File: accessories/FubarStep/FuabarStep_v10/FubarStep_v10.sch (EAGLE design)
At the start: 10 parts, among them IC1 7805, X1 DC21MMX

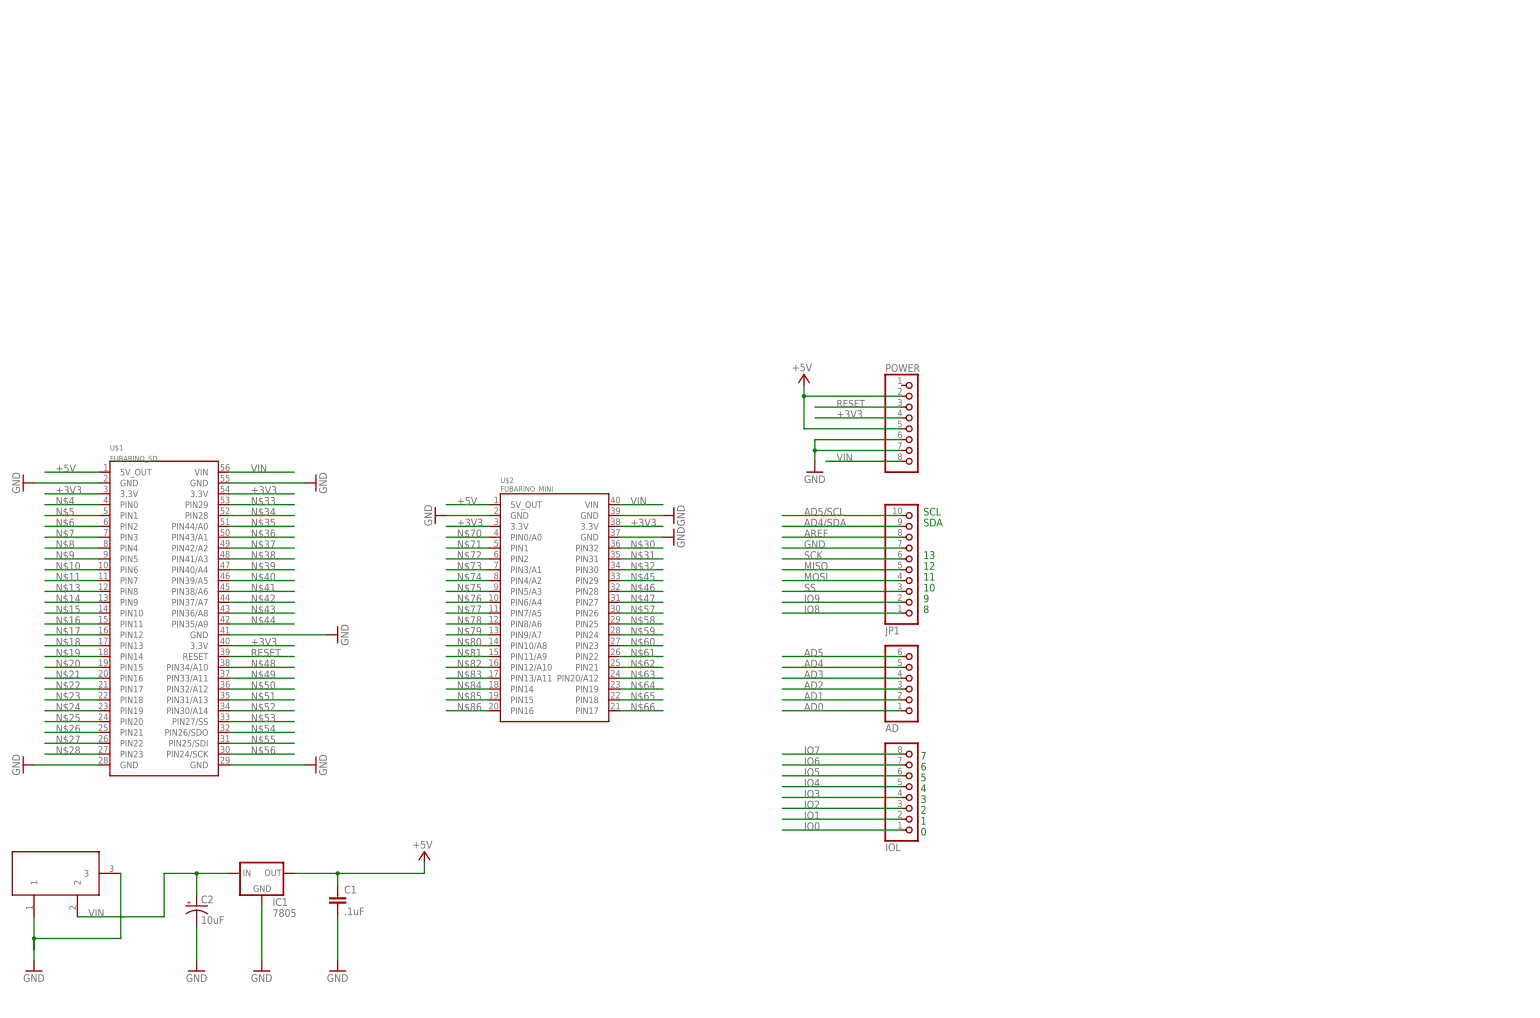
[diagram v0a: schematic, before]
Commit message: More work.
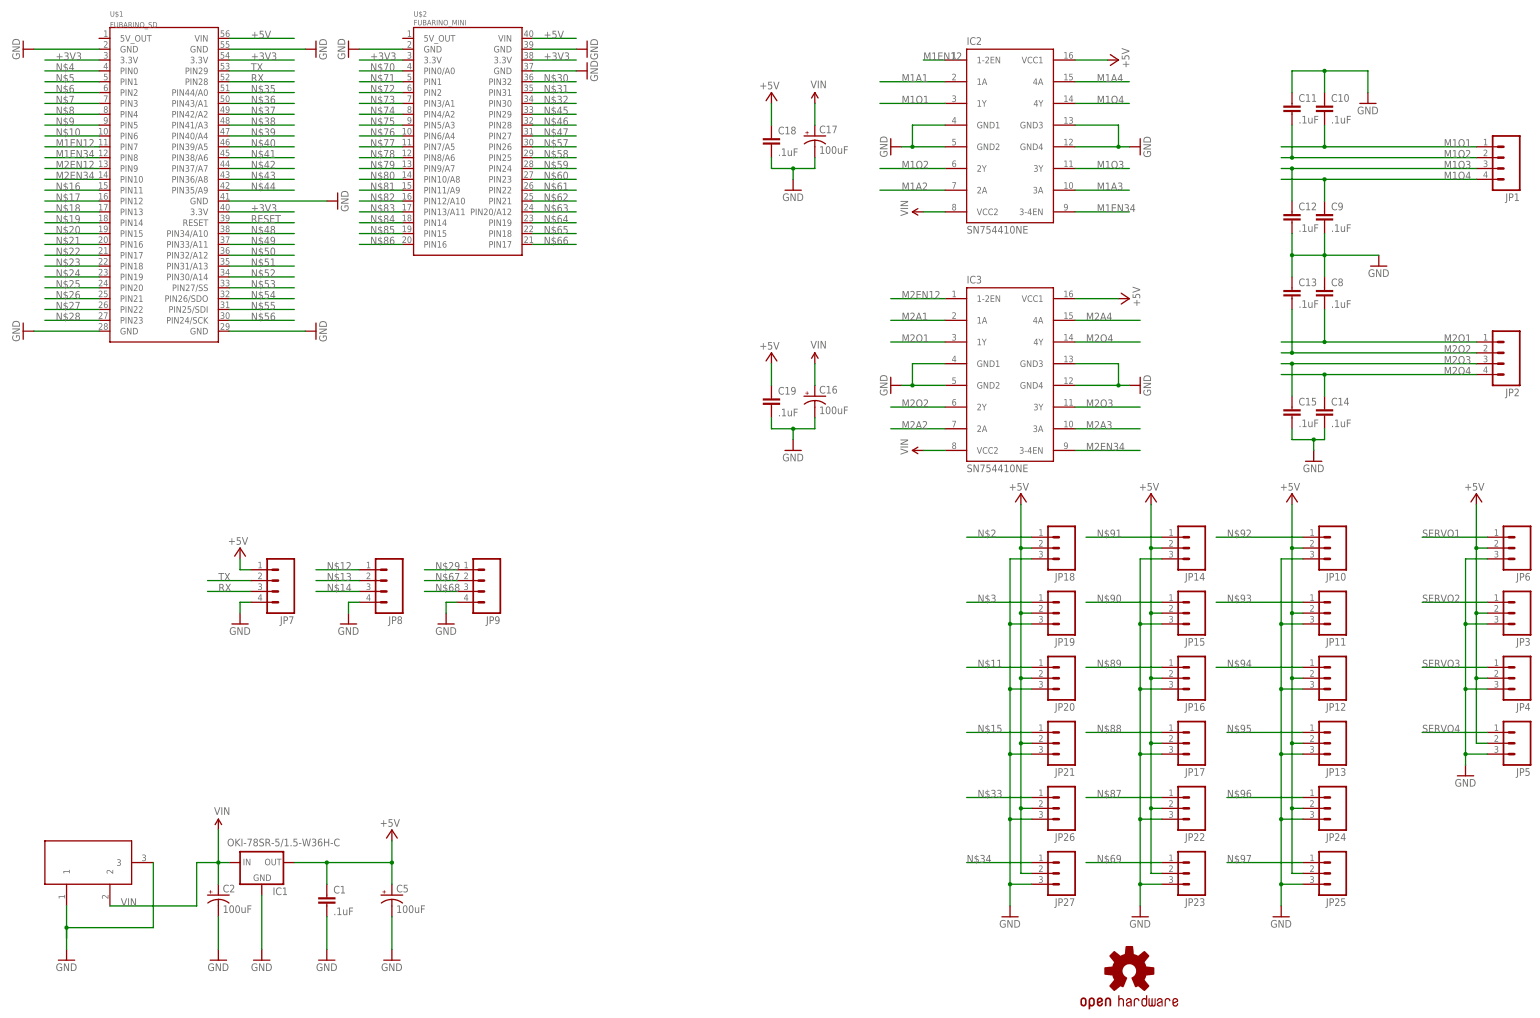
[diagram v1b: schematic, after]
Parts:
- removed AD: (no value), pinhead:PINHD-1X6
- removed IOL, POWER: (no value), pinhead:PINHD-1X8
- added C10, C11, C12, C13, C14, C15, C18, C19, C8, C9: .1uF, SparkFun-Capacitors:CAPPTH
- added C16, C17, C5: 100uF, SparkFun-Capacitors:CAP_POLPTH1
- added IC2, IC3: SN754410NE, texas:L293E
- added JP10, JP11, JP12, JP13, JP14, JP15, JP16, JP17, JP18, JP19, JP20, JP21, JP22, JP23, JP24, JP25, JP26, JP27, JP3, JP4, JP5, JP6: (no value), SparkFun-Connectors:M03LOCK
- added JP2: (no value), SparkFun-Connectors:M04SCREW_LOCK
- added JP7, JP8, JP9: (no value), SparkFun-Connectors:M04LOCK
- added LOGO1: OSHW-LOGOM, SparkFun-Aesthetics:OSHW-LOGOM
- C2: value 10uF -> 100uF; device SparkFun-Capacitors:CAP_POLPTH2 -> SparkFun-Capacitors:CAP_POLPTH1
- IC1: value 7805 -> OKI-78SR-5/1.5-W36H-C
- JP1: device pinhead:PINHD-1X10 -> SparkFun-Connectors:M04SCREW_LOCK
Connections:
- removed net AD0: AD.1
- removed net AD1: AD.2
- removed net AD2: AD.3
- removed net AD3: AD.4
- removed net AD4: AD.5
- removed net AD4/SDA: JP1.9
- removed net AD5: AD.6
- removed net AD5/SCL: JP1.10
- removed net AREF: JP1.8
- removed net IO0: IOL.1
- removed net IO1: IOL.2
- removed net IO2: IOL.3
- removed net IO3: IOL.4
- removed net IO4: IOL.5
- removed net IO5: IOL.6
- removed net IO6: IOL.7
- removed net IO7: IOL.8
- removed net IO8: JP1.1
- removed net IO9: JP1.2
- removed net MISO: JP1.5
- removed net MOSI: JP1.4
- removed net SCK: JP1.6
- removed net SS: JP1.3
- new net M1A1: IC2.1A
- new net M1A2: IC2.2A
- new net M1A3: IC2.3A
- new net M1A4: IC2.4A
- new net M1EN12: IC2.1-2EN, U$1.PIN7
- new net M1EN34: IC2.3-4EN, U$1.PIN8
- new net M1O1: C10.2, IC2.1Y, JP1.1
- new net M1O2: C11.2, IC2.2Y, JP1.2
- new net M1O3: C12.1, IC2.3Y, JP1.3
- new net M1O4: C9.1, IC2.4Y, JP1.4
- new net M2A1: IC3.1A
- new net M2A2: IC3.2A
- new net M2A3: IC3.3A
- new net M2A4: IC3.4A
- new net M2EN12: IC3.1-2EN, U$1.PIN9
- new net M2EN34: IC3.3-4EN, U$1.PIN10
- new net M2O1: C8.2, IC3.1Y, JP2.1
- new net M2O2: C13.2, IC3.2Y, JP2.2
- new net M2O3: C15.1, IC3.3Y, JP2.3
- new net M2O4: C14.1, IC3.4Y, JP2.4
- new net N$12: JP8.1
- new net N$2: JP18.1
- new net N$29: JP9.1
- new net N$3: JP19.1
- new net N$67: JP9.2
- new net N$68: JP9.3
- new net N$69: JP23.1
- new net N$87: JP22.1
- new net N$88: JP17.1
- new net N$89: JP16.1
- new net N$90: JP15.1
- new net N$91: JP14.1
- new net N$92: JP10.1
- new net N$93: JP11.1
- new net N$94: JP12.1
- new net N$95: JP13.1
- new net N$96: JP24.1
- new net N$97: JP25.1
- new net RX: JP7.3, U$1.PIN28
- new net SERVO1: JP6.1
- new net SERVO2: JP3.1
- new net SERVO3: JP4.1
- new net SERVO4: JP5.1
- new net TX: JP7.2, U$1.PIN29
- net +3V3: no longer POWER.4
- net +5V: now also C18.1, C19.1, C5.+, IC2.VCC1, IC3.VCC1, JP10.2, JP11.2, JP12.2, JP13.2, JP14.2, JP15.2, JP16.2, JP17.2, JP18.2, JP19.2, JP20.2, JP21.2, JP22.2, JP23.2, JP24.2, JP25.2, JP26.2, JP27.2, JP3.2, JP4.2, JP5.2, JP6.2, JP7.1, U$1.VIN, U$2.VIN; no longer POWER.2, POWER.5, U$1.5V_OUT, U$2.5V_OUT
- net GND: now also C10.1, C11.1, C12.2, C13.1, C14.2, C15.2, C16.-, C17.-, C18.2, C19.2, C5.-, C8.1, C9.2, IC2.GND1, IC2.GND2, IC2.GND3, IC2.GND4, IC3.GND1, IC3.GND2, IC3.GND3, IC3.GND4, JP10.3, JP11.3, JP12.3, JP13.3, JP14.3, JP15.3, JP16.3, JP17.3, JP18.3, JP19.3, JP20.3, JP21.3, JP22.3, JP23.3, JP24.3, JP25.3, JP26.3, JP27.3, JP3.3, JP4.3, JP5.3, JP6.3, JP7.4, JP8.4, JP9.4; no longer JP1.7, POWER.6, POWER.7
- net N$11: now also JP20.1; no longer U$1.PIN7
- net N$13: now also JP8.2; no longer U$1.PIN8
- net N$14: now also JP8.3; no longer U$1.PIN9
- net N$15: now also JP21.1; no longer U$1.PIN10
- net N$33: now also JP26.1; no longer U$1.PIN29
- net N$34: now also JP27.1; no longer U$1.PIN28
- net RESET: no longer POWER.3
- net VIN: now also C16.+, C17.+, IC2.VCC2, IC3.VCC2; no longer POWER.8, U$1.VIN, U$2.VIN
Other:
- note added: "Fubarino Stepper Shield"
- note removed: "0"
- note removed: "1"
- note removed: "10"
- note removed: "11"
- note removed: "12"
- note removed: "13"
- note removed: "2"
- note removed: "3"
- note removed: "4"
- note removed: "5"
- note removed: "6"
- note removed: "7"
- note removed: "8"
- note removed: "9"
- note removed: "Fubarino Arduino Uno Adapter Board"
- note removed: "SCL"
- note removed: "SDA"
- moved on the sheet: C1, C2, IC1, U$1, U$2
